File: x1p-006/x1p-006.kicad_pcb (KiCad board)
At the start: 2 copper layers, 26 x 32.6 mm, 18 parts, among them U1 AD24C02, U2 AQY212EHAX, U3 AQY212EHAX

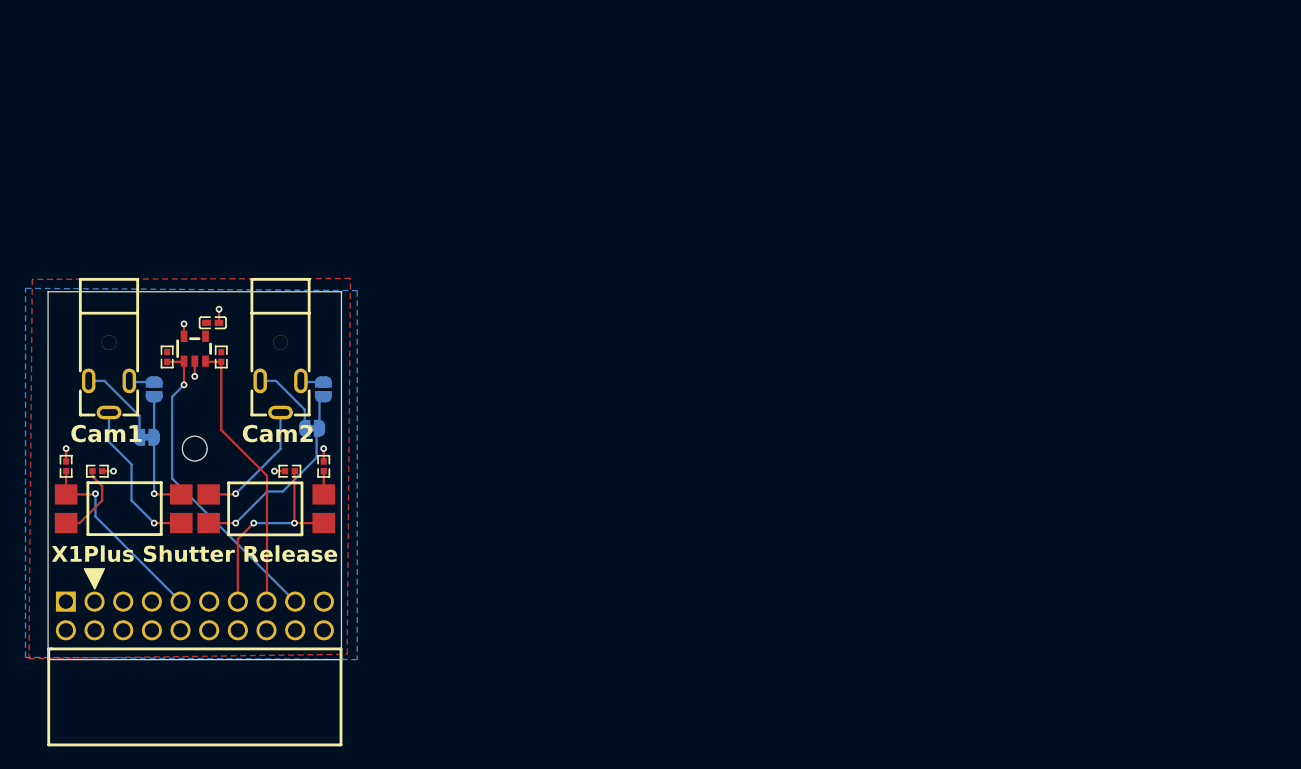
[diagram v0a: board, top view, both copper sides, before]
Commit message: x1p-006: adjust layout to homogenize
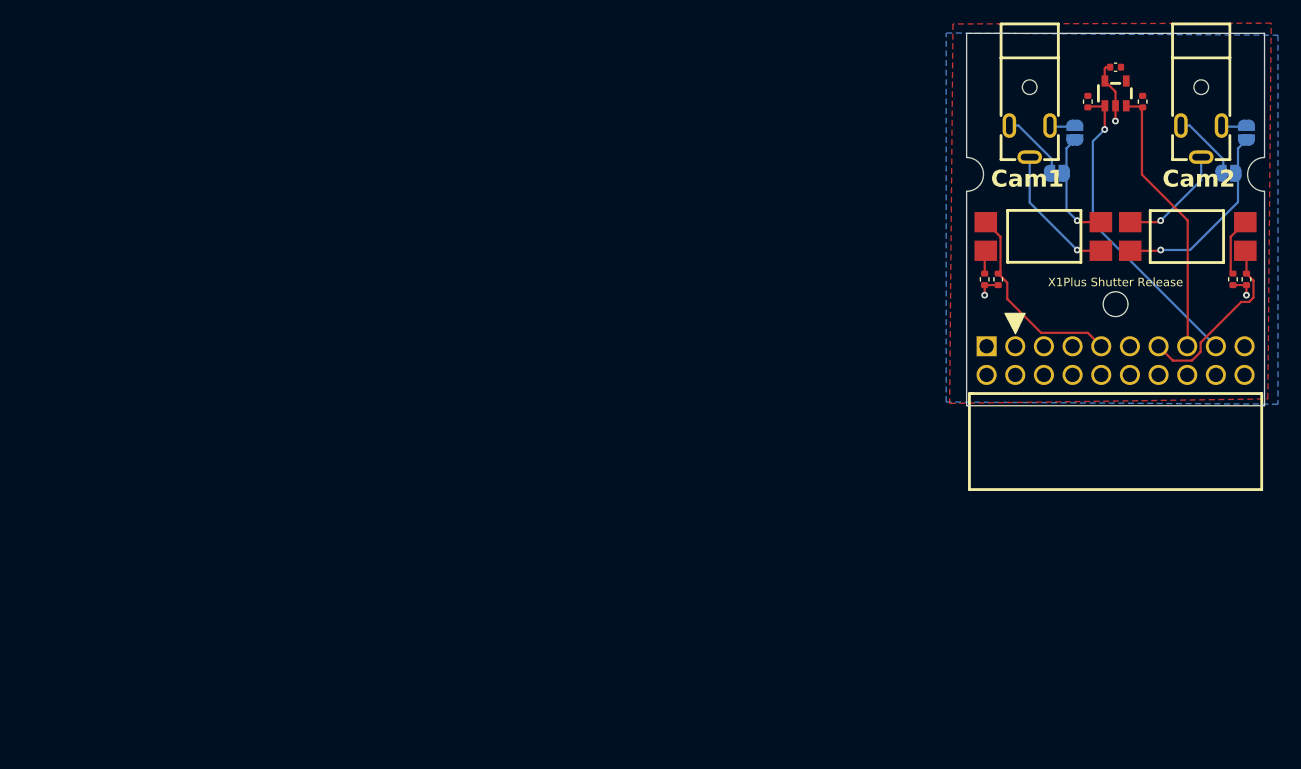
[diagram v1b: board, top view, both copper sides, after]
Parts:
- C1: footprint x1p-006:C0402 -> Capacitor_SMD:C_0402_1005Metric
- R1, R2, R3, R4, R5, R6: footprint x1p-006:R0402 -> Resistor_SMD:R_0402_1005Metric
- moved R6 86.5 mm to (161.6, 92.8), turned to 90 degrees
- moved U3 85.2 mm to (156.4, 89.0)
- moved U2 85.0 mm to (143.6, 89.0)
- moved JP4 84.9 mm to (161.6, 79.8)
- moved R2 84.7 mm to (152.4, 77.0)
- moved JP2 84.7 mm to (146.4, 79.8)
- moved U1 84.7 mm to (150.0, 76.3)
- moved CAM2 84.7 mm to (157.6, 80.6)
- moved HDR1 84.7 mm to (150.0, 100.0)
- moved CAM1 84.7 mm to (142.4, 80.6)
- moved R1 84.7 mm to (147.5, 77.0)
- moved JP3 84.3 mm to (160.0, 83.4)
- moved R5 84.2 mm to (139.6, 92.8), turned to 90 degrees
- moved JP1 84.0 mm to (144.8, 83.4)
- moved C1 83.1 mm to (150.0, 74.0), turned to 180 degrees
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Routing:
- net Net-(U2-K): track 6.98 -> 2.77 mm
- net Net-(U3-K): track 2.06 -> 5.18 mm
- net GND: track 7.87 -> 9.75 mm, vias 7 -> 3
- net Net-(U2-S1): track 13.9 -> 12.1 mm
- net LD5: track 18.4 -> 16.9 mm, vias 2 -> 0
- net Net-(JP1-B): track 7.68 -> 6.26 mm
- net Net-(U3-S1): track 11.3 -> 9.87 mm
- net Net-(JP1-A): track 11.1 -> 10.0 mm
- net LD3: track 17.4 -> 17.8 mm, vias 1 -> 0
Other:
- board size 26 x 32.6 mm -> 26.4 x 33 mm
- board text added: "X1P-006-B02"
- board text removed: "X1P-006-B01"

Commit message: reduce overall BOM on panels, load manufacturer and MPN in
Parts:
- C1: value 0.1uf -> 0.1uF
- HDR1: value 220R-2*10P H=8.5MM Ytype Gold-plated black -> B-2200R20P-B120
- R1, R2, R5, R6: value 3.3k -> 2.2k
